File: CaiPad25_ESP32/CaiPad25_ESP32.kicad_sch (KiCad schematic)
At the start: 27 parts, among them J1 OLED_128x64, U1 ESP32_DevKit_V1_DOIT

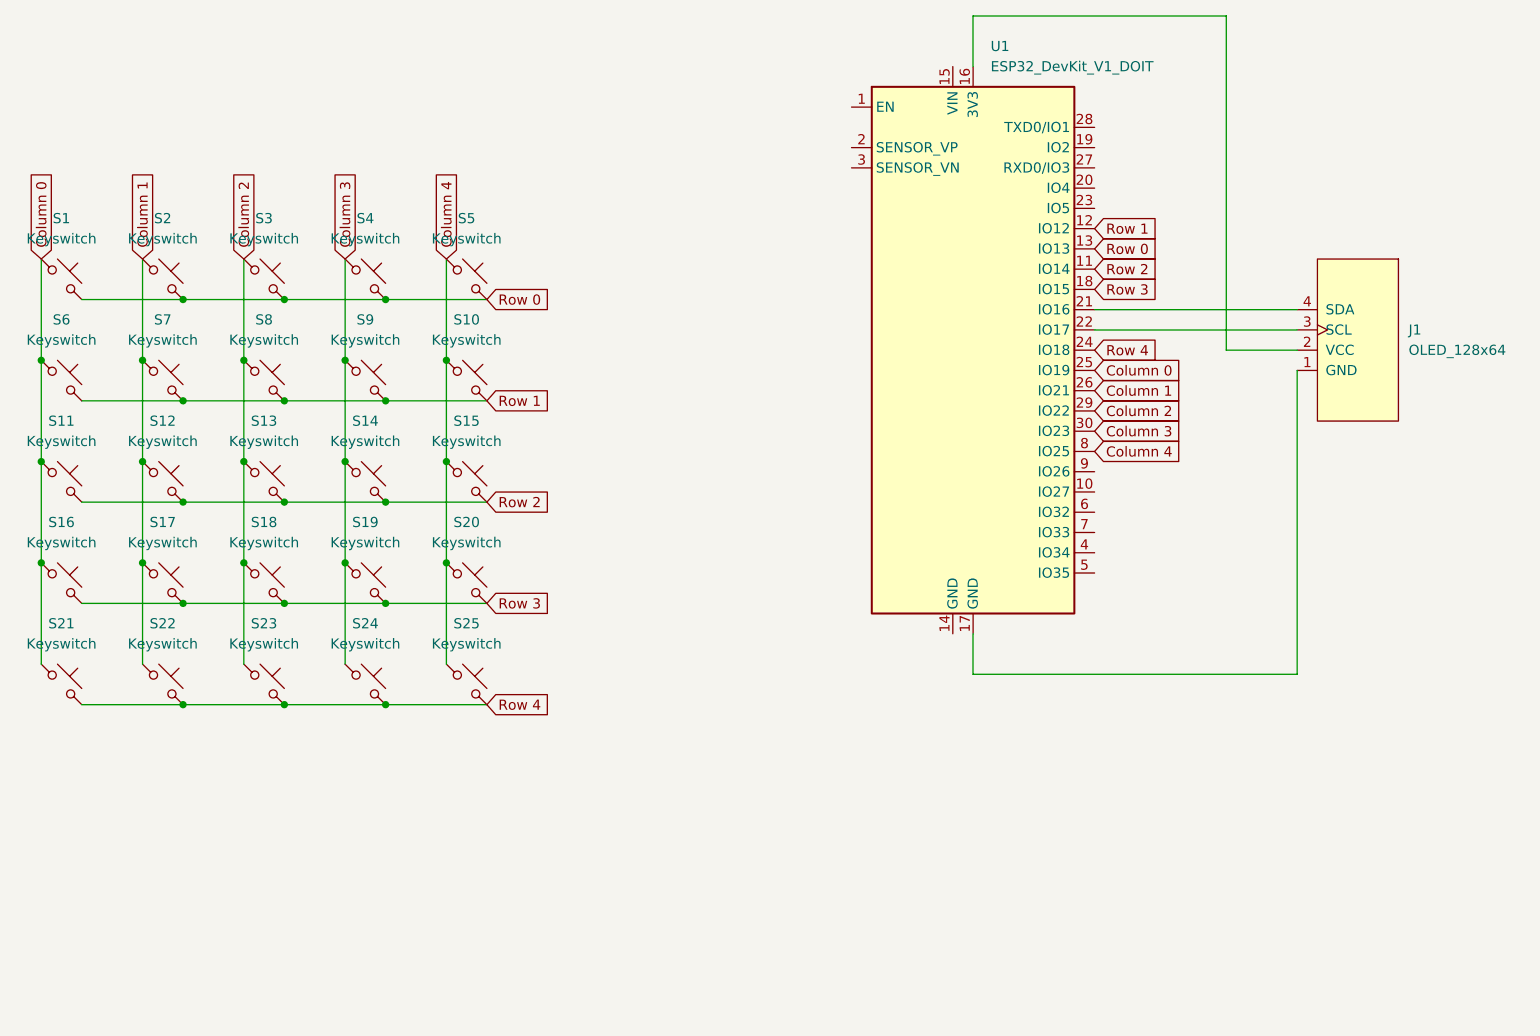
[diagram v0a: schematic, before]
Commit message: update on CaiPad25_ESP32
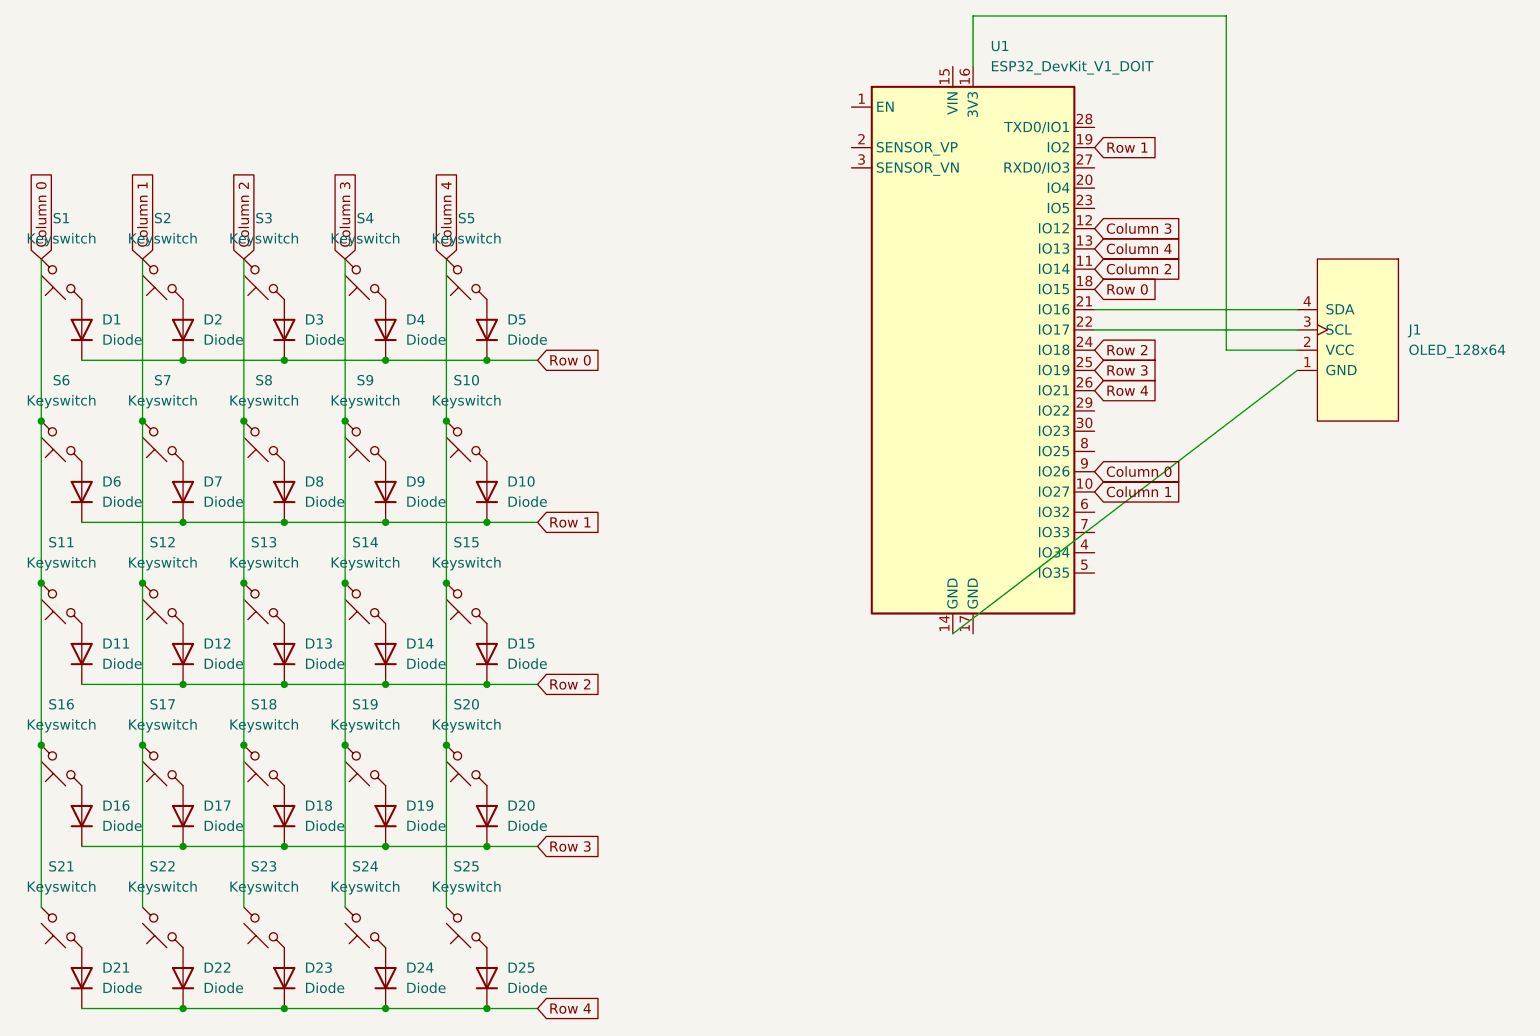
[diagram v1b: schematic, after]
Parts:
- added D1, D10, D11, D12, D13, D14, D15, D16, D17, D18, D19, D2, D20, D21, D22, D23, D24, D25, D3, D4, D5, D6, D7, D8, D9: Diode, ScottoKeebs_Components:Diode_DO-35, symbol ScottoKeebs:Placeholder_Diode
- S1, S10, S11, S12, S13, S14, S15, S16, S17, S18, S19, S2, S20, S21, S22, S23, S24, S25, S3, S4, S5, S6, S7, S8, S9: footprint ScottoKeebs_MX:MX_PCB_1.00u -> Button_Switch_Keyboard:SW_Cherry_MX_1.00u_PCB
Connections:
- net Column 0: now also S1.2, S11.2, S16.2, S21.2, S6.2, U1.9 (IO26); no longer S1.1, S11.1, S16.1, S21.1, S6.1, U1.25 (IO19)
- net Column 1: now also S12.2, S17.2, S2.2, S22.2, S7.2, U1.10 (IO27); no longer S12.1, S17.1, S2.1, S22.1, S7.1, U1.26 (IO21)
- net Column 2: now also S13.2, S18.2, S23.2, S3.2, S8.2, U1.11 (IO14); no longer S13.1, S18.1, S23.1, S3.1, S8.1, U1.29 (IO22)
- net Column 3: now also S14.2, S19.2, S24.2, S4.2, S9.2, U1.12 (IO12); no longer S14.1, S19.1, S24.1, S4.1, S9.1, U1.30 (IO23)
- net Column 4: now also S10.2, S15.2, S20.2, S25.2, S5.2, U1.13 (IO13); no longer S10.1, S15.1, S20.1, S25.1, S5.1, U1.8 (IO25)
- net Row 0: now also U1.18 (IO15), D1.1 (K), D2.1 (K), D3.1 (K), D4.1 (K), D5.1 (K); no longer S1.2, S2.2, S3.2, S4.2, S5.2, U1.13 (IO13)
- net Row 1: now also U1.19 (IO2), D10.1 (K), D6.1 (K), D7.1 (K), D8.1 (K), D9.1 (K); no longer S10.2, S6.2, S7.2, S8.2, S9.2, U1.12 (IO12)
- net Row 2: now also U1.24 (IO18), D11.1 (K), D12.1 (K), D13.1 (K), D14.1 (K), D15.1 (K); no longer S11.2, S12.2, S13.2, S14.2, S15.2, U1.11 (IO14)
- net Row 3: now also U1.25 (IO19), D16.1 (K), D17.1 (K), D18.1 (K), D19.1 (K), D20.1 (K); no longer S16.2, S17.2, S18.2, S19.2, S20.2, U1.18 (IO15)
- net Row 4: now also U1.26 (IO21), D21.1 (K), D22.1 (K), D23.1 (K), D24.1 (K), D25.1 (K); no longer S21.2, S22.2, S23.2, S24.2, S25.2, U1.24 (IO18)
- net at U1.14 (GND): now also J1.1 (GND)
- net at U1.17 (GND): no longer J1.1 (GND)
- new net: D16.2 (A), S16.1
- new net: D18.2 (A), S18.1
- new net: D12.2 (A), S12.1
- new net: D4.2 (A), S4.1
- new net: D13.2 (A), S13.1
- new net: D23.2 (A), S23.1
- new net: D7.2 (A), S7.1
- new net: D1.2 (A), S1.1
- new net: D19.2 (A), S19.1
- new net: D8.2 (A), S8.1
- new net: D9.2 (A), S9.1
- new net: D2.2 (A), S2.1
- new net: D21.2 (A), S21.1
- new net: D17.2 (A), S17.1
- new net: D6.2 (A), S6.1
- new net: D25.2 (A), S25.1
- new net: D15.2 (A), S15.1
- new net: D10.2 (A), S10.1
- new net: D22.2 (A), S22.1
- new net: D20.2 (A), S20.1
- new net: D3.2 (A), S3.1
- new net: D24.2 (A), S24.1
- new net: D5.2 (A), S5.1
- new net: D11.2 (A), S11.1
- new net: D14.2 (A), S14.1
